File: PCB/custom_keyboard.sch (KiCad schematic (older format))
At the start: 393 parts, among them IC1 FE2.1, J1 USB_A, J2 USB_A, J3 USB_A, J4 Conn_01x08_Male, SW1 SW_Push, U1 PRTR5V0U2X, U2 24LC02, U3 PRTR5V0U2X, U4 PRTR5V0U2X, U5 PRTR5V0U2X, U6 PRTR5V0U2X, U7 PRTR5V0U2X, U8 PRTR5V0U2X, U9 AT90USB646-MU, Y1 12MHz, Y2 16MHz

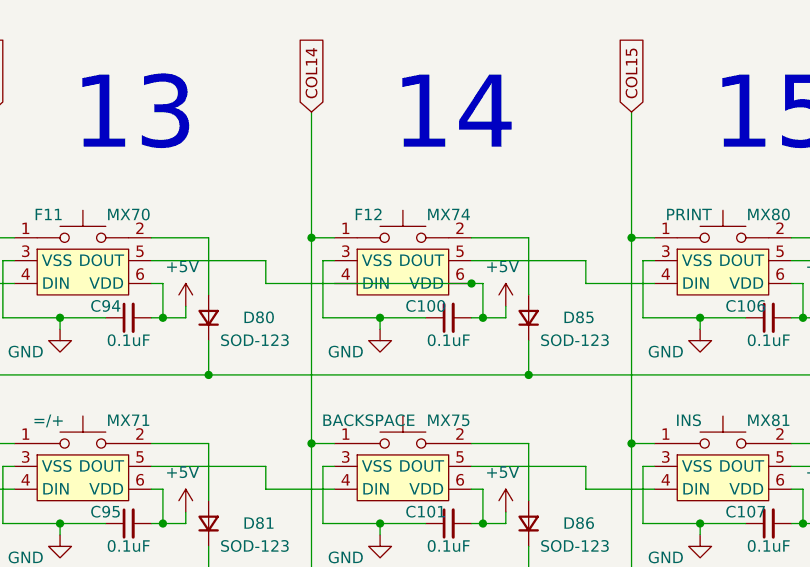
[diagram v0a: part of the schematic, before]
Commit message: Routed lights
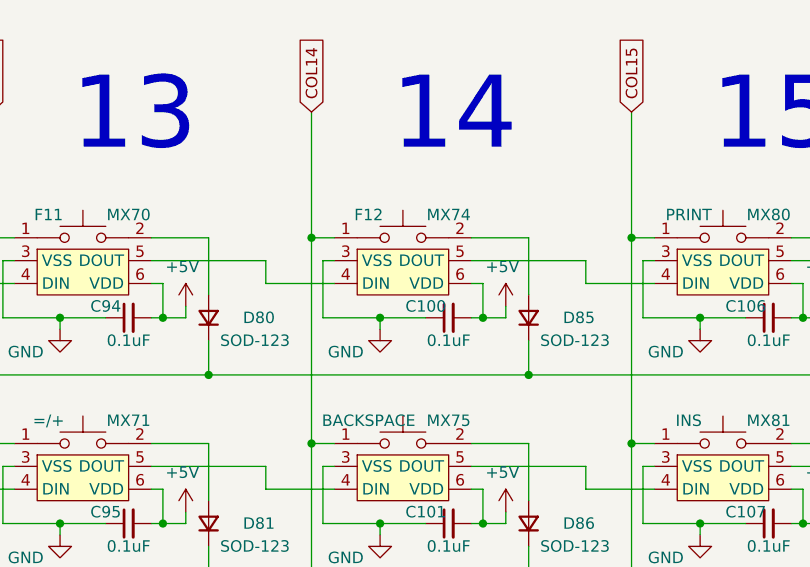
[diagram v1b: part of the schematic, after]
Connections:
- net +5V: no longer MX70.5 (DOUT), MX74.4 (DIN)
- new net: MX70.5 (DOUT), MX74.4 (DIN)
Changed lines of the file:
@@
 Wire Wire Line
 	10600 3900 10500 3900
-Connection ~ 23800 4100
-Wire Wire Line
-	23800 4100 23200 4100
 Wire Wire Line
 	20400 6600 20300 6600
